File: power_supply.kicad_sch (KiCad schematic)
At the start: 33 parts, among them U1 RP115H331D, U3 RP115H181D

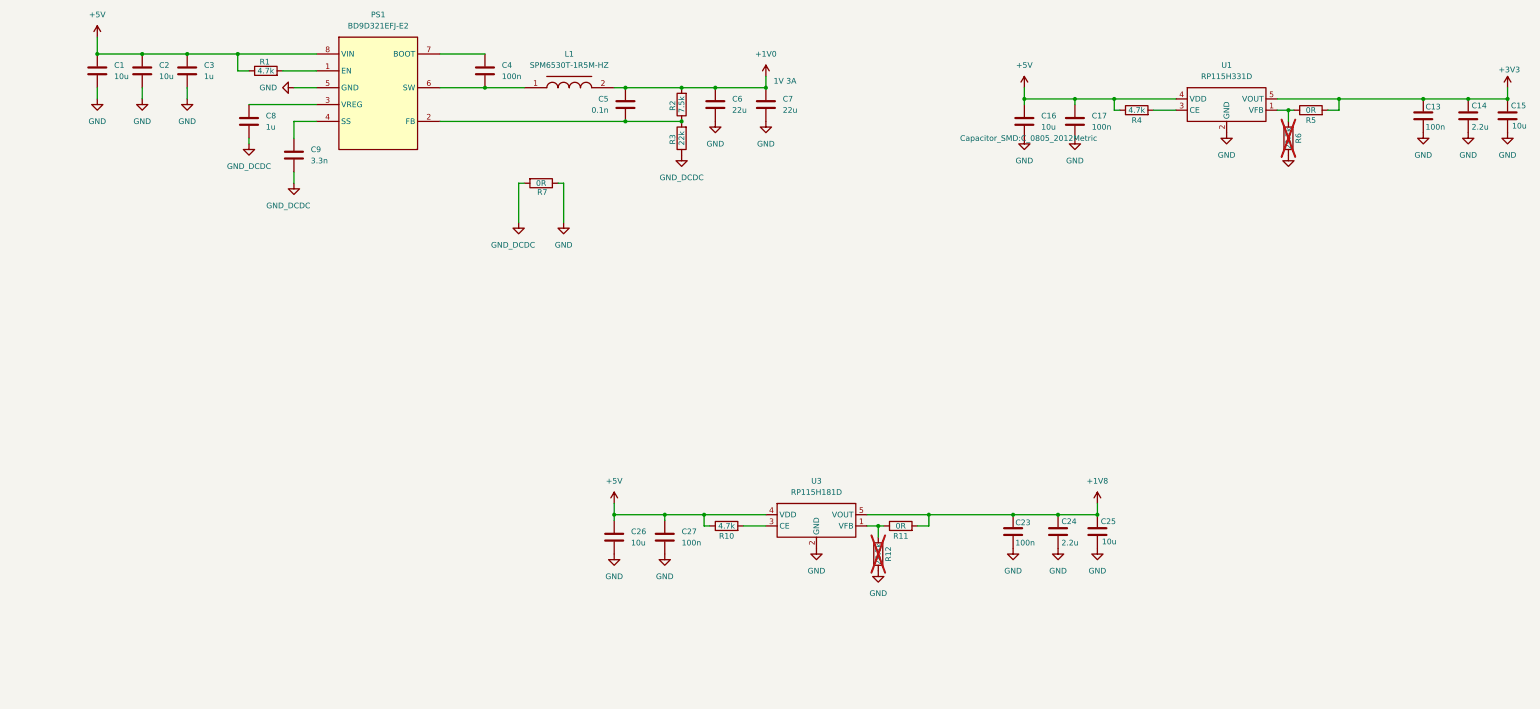
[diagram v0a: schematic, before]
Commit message: relay unit
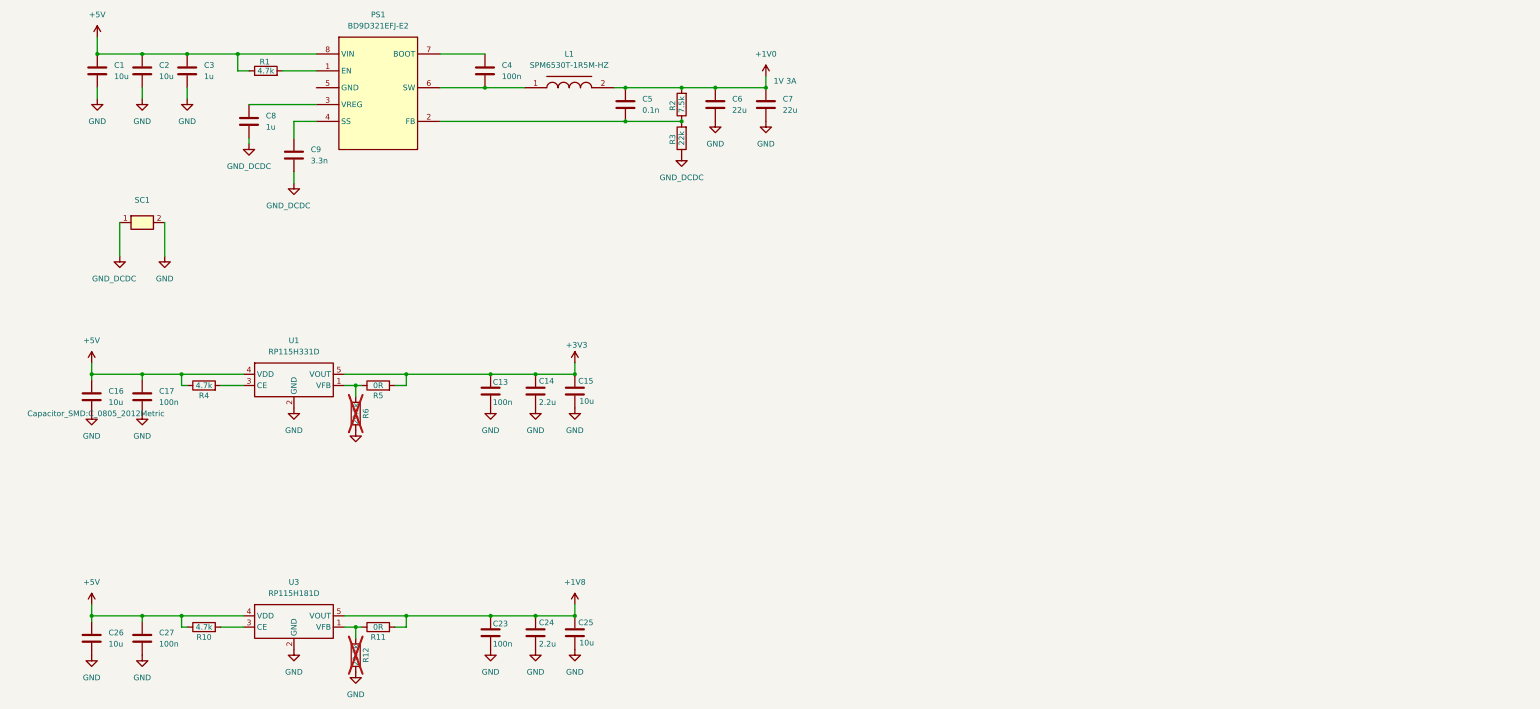
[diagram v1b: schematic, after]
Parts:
- removed R7: 0R, Resistor_SMD:R_0603_1608Metric, symbol Device:R
- added SC1: ~, house:short_conn, symbol house:short_conn
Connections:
- net GND: now also SC1.2; no longer PS1.5 (GND)
- net GND_DCDC: now also SC1.1
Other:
- moved on the sheet: C13, C14, C15, C16, C17, C23, C24, C25, C26, C27, R10, R11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
